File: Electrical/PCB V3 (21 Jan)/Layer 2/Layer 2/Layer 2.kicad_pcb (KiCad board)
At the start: 2 copper layers, 180 x 172.1 mm, 73 parts, among them Q1 AON6354, Q2 AON6354, Q3 AON6354, Q4 AON6354, SW1 SW_Nidec_CAS-120A1, U2 LM2596S-3.3, U3 VNH5019ATR-E, U4 XT30UPB-M, U5 XT30UPB-M, U6 VNH5019ATR-E, U7 VNH5019ATR-E, U8 VNH5019ATR-E, U9 XT30UPB-M

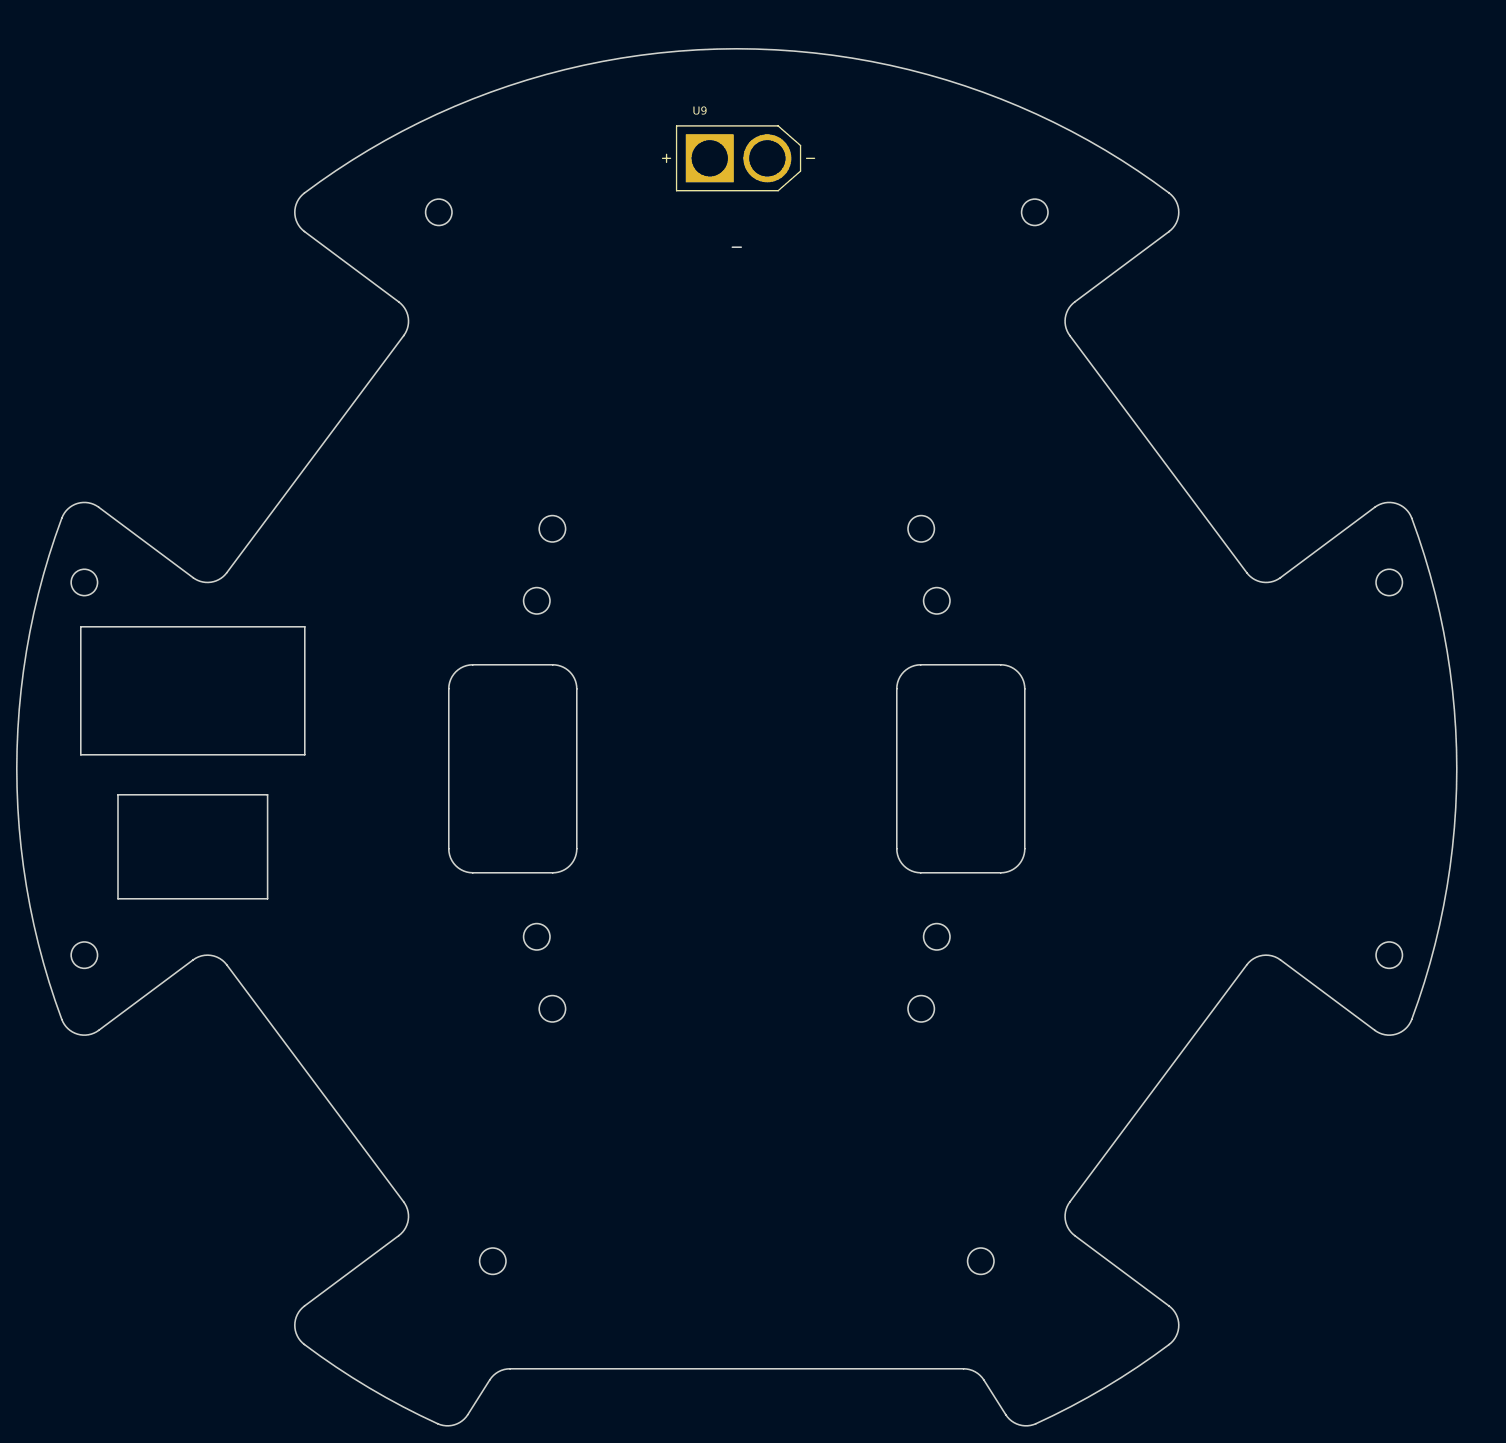
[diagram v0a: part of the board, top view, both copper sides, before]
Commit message: lmao cx
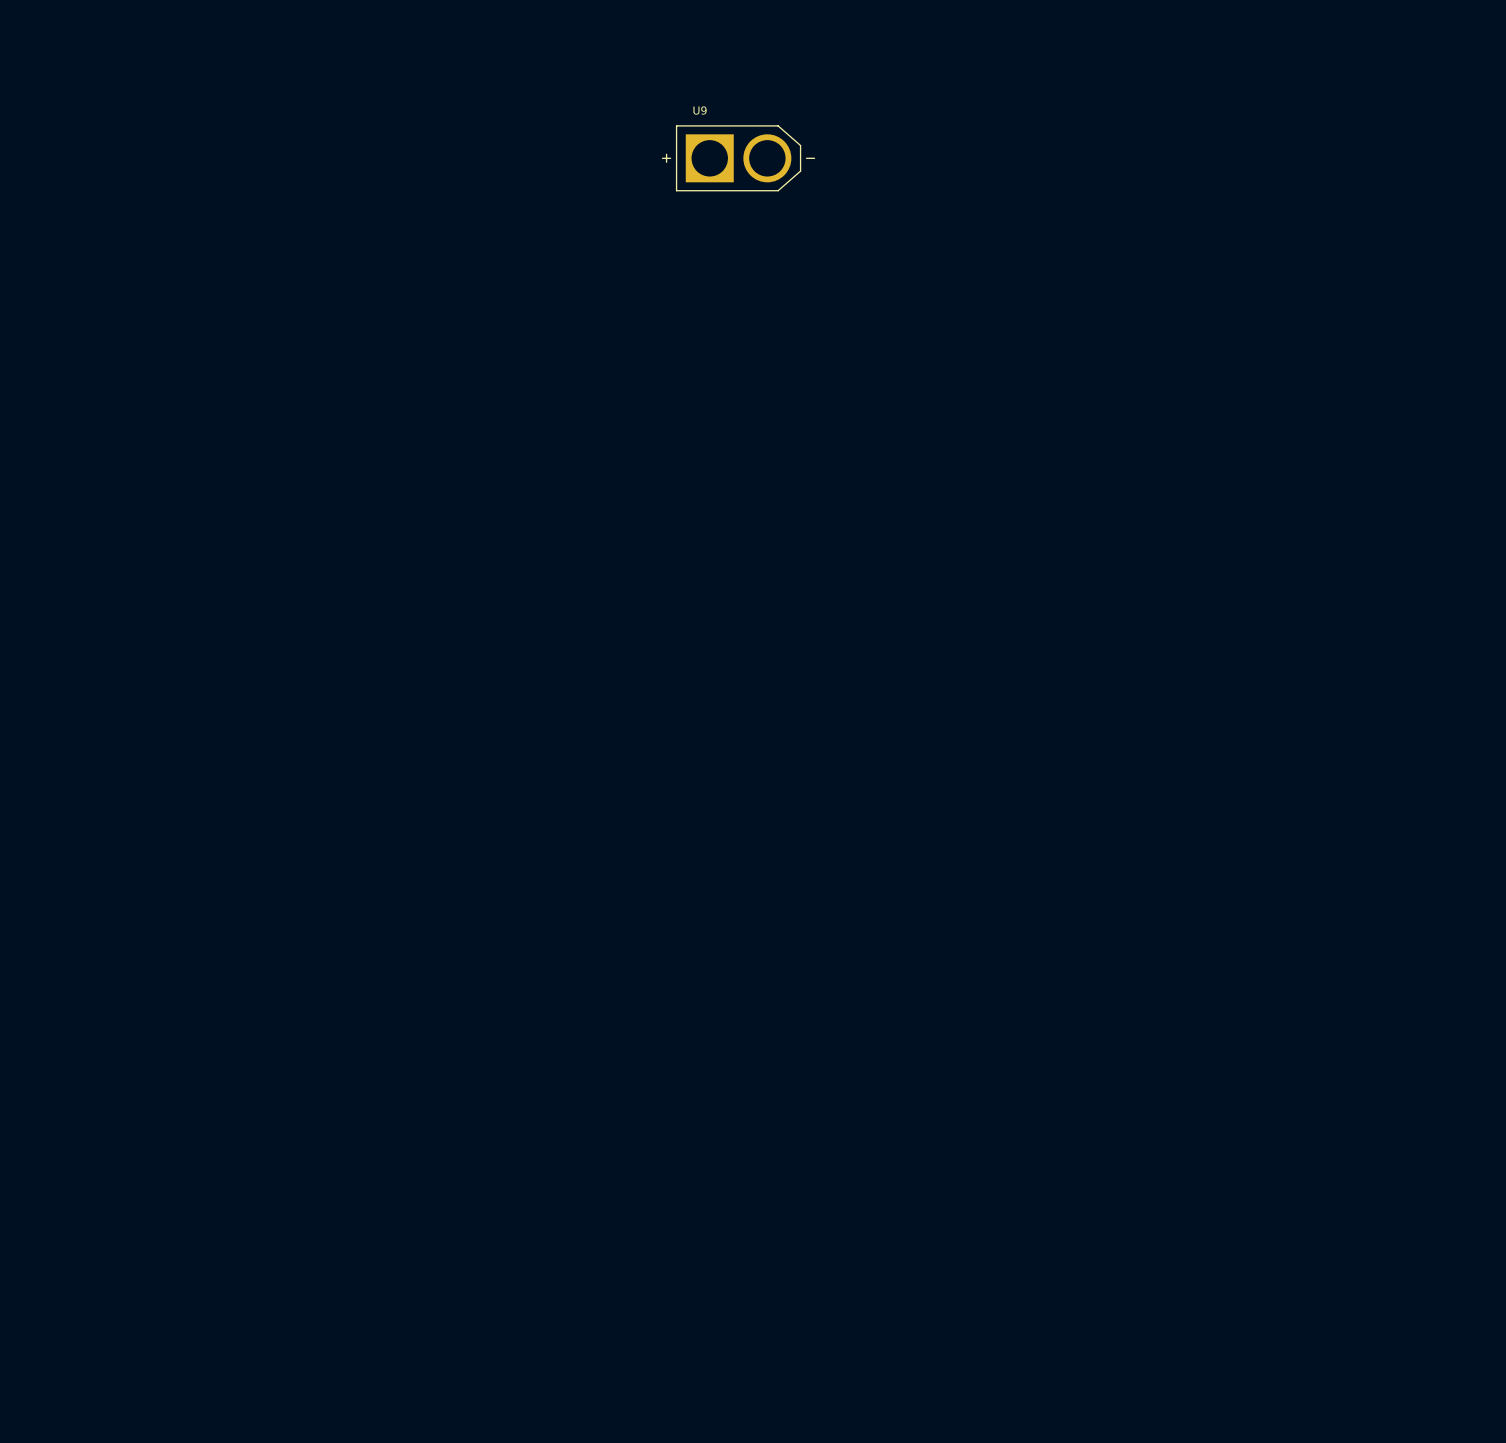
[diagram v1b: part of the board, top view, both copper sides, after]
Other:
- board outline removed
